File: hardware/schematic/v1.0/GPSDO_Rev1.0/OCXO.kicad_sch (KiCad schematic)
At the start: 47 parts, among them U10 SN74LVC1T45DBVR, U2 LMK1C1103PWR, U3 TMP117AIDRVR, U5 OCXO_20x20mm, U7 OCXO_25.4x25.4mm, U8 REF5040, U9 OPA388IDR

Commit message: sch update
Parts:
- C1, C16, C18, C22, C24, C4, C5: symbol GPSDO_Rev1.0:C -> GPSDO_Rev1.0:C__C_0402_1005Metric
- C11: footprint Capacitor_SMD:C_0402_1005Metric -> GPSDO_Rev1.0:C_0402_1005Metric; symbol Device:C -> GPSDO_Rev1.0:C__C_0402_1005Metric
- C56, C57, C58: footprint Capacitor_SMD:C_0603_1608Metric -> GPSDO_Rev1.0:C_0603_1608Metric; symbol Device:C -> GPSDO_Rev1.0:C
- R12, R13, R15, R16, R35, R37, R4: symbol GPSDO_Rev1.0:R -> GPSDO_Rev1.0:R__R_0402_1005Metric
- R28, R29: footprint Resistor_SMD:R_0603_1608Metric -> GPSDO_Rev1.0:R_0603_1608Metric; symbol Device:R -> GPSDO_Rev1.0:R
- R5: symbol GPSDO_Rev1.0:R -> GPSDO_Rev1.0:R__R_0805_2012Metric
- R6: symbol GPSDO_Rev1.0:R -> GPSDO_Rev1.0:R__C_0603_1608Metric
- TP1, TP2: footprint TestPoint:TestPoint_Pad_D1.0mm -> GPSDO_Rev1.0:TestPoint_Pad_D1.0mm; symbol Connector:TestPoint -> GPSDO_Rev1.0:TestPoint
- U8: footprint JLCImport:REF5040 -> GPSDO_Rev1.0:REF5040; symbol JLCImport:REF5040 -> GPSDO_Rev1.0:REF5040

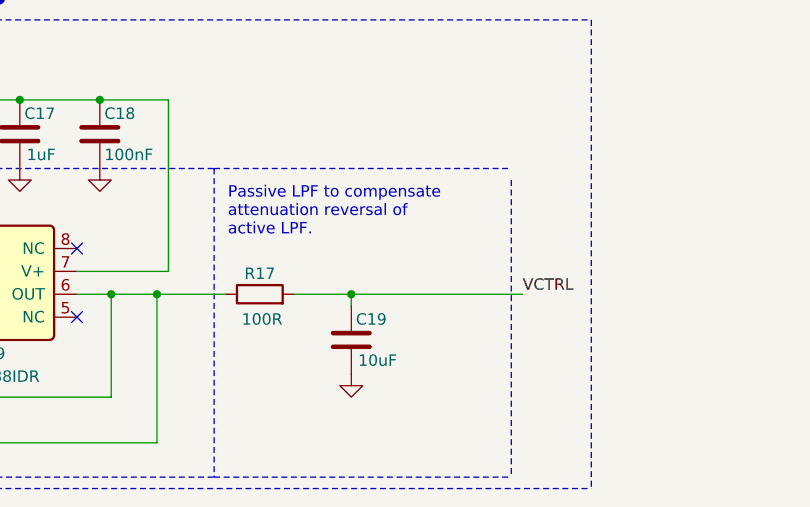
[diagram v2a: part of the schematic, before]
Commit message: sch update
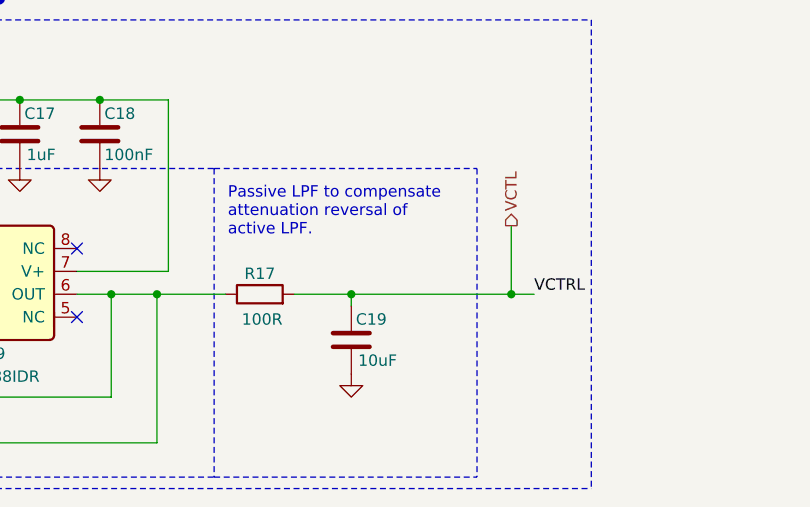
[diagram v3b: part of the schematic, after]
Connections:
- net VCTRL renamed VCTL
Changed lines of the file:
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@@
+	)
+	(junction
+		(at 246.38 35.56)
+		(diameter 0)
+		(color 0 0 0 0)
+	)
+	(junction
+		(at 78.74 111.76)
+		(diameter 0)
+		(color 0 0 0 0)
+	)
+	(junction
+		(at 67.31 111.76)
+		(diameter 0)
+		(color 0 0 0 0)
+	)
+	(junction
+		(at 205.74 44.45)
+		(diameter 0)
+		(color 0 0 0 0)
+	)
+	(junction
+		(at 72.39 173.99)
+		(diameter 0)
+		(color 0 0 0 0)
+	)
+	(junction
+		(at 120.65 173.99)
+		(diameter 0)
+		(color 0 0 0 0)
+	)
+	(junction
+		(at 201.93 57.15)
+		(diameter 0)
+		(color 0 0 0 0)
+	)
+	(junction
+		(at 83.82 50.8)
+		(diameter 0)
+		(color 0 0 0 0)
+	)
+	(junction
+		(at 142.24 111.76)
+		(diameter 0)
+		(color 0 0 0 0)
+	)
+	(junction
+		(at 92.71 111.76)
+		(diameter 0)
+		(color 0 0 0 0)
+	)
+	(junction
+		(at 165.1 173.99)
+		(diameter 0)
+		(color 0 0 0 0)
+	)
+	(junction
+		(at 87.63 173.99)
+		(diameter 0)
+		(color 0 0 0 0)
+	)
+	(junction
+		(at 110.49 152.4)
+		(diameter 0)
+		(color 0 0 0 0)
+	)
+	(junction
+		(at 246.38 46.99)
+		(diameter 0)
+		(color 0 0 0 0)
+	)
+	(junction
+		(at 46.99 50.8)
+		(diameter 0)
+		(color 0 0 0 0)
+	)
+	(junction
+		(at 138.43 102.87)
+		(diameter 0)
+		(color 0 0 0 0)
+	)
+	(junction
+		(at 129.54 111.76)
+		(diameter 0)
+		(color 0 0 0 0)
+	)
+	(junction
+		(at 157.48 97.79)
+		(diameter 0)
+		(color 0 0 0 0)
+	)
+	(junction
+		(at 134.62 111.76)
+		(diameter 0)
+		(color 0 0 0 0)
+	)
+	(junction
+		(at 125.73 173.99)
+		(diameter 0)
+		(color 0 0 0 0)
+	)
+	(junction
+		(at 198.12 44.45)
+		(diameter 0)
+		(color 0 0 0 0)
+	)
+	(junction
+		(at 25.4 173.99)
+		(diameter 0)
+		(color 0 0 0 0)
+	)
+	(junction
+		(at 157.48 106.68)
+		(diameter 0)
+		(color 0 0 0 0)
+	)
+	(junction
+		(at 49.53 151.13)
+		(diameter 0)
+		(color 0 0 0 0)
+	)
+	(junction
+		(at 205.74 57.15)
+		(diameter 0)
+		(color 0 0 0 0)
 	)
 	(junction
 		(at 147.32 173.99)
-		(diameter 0)
-		(color 0 0 0 0)
-	)
-	(junction
-		(at 246.38 35.56)
-		(diameter 0)
-		(color 0 0 0 0)
-	)
-	(junction
-		(at 78.74 111.76)
-		(diameter 0)
-		(color 0 0 0 0)
-	)
-	(junction
-		(at 67.31 111.76)
-		(diameter 0)
-		(color 0 0 0 0)
-	)
-	(junction
-		(at 205.74 44.45)
-		(diameter 0)
-		(color 0 0 0 0)
-	)
-	(junction
-		(at 72.39 173.99)
-		(diameter 0)
-		(color 0 0 0 0)
-	)
-	(junction
-		(at 120.65 173.99)
-		(diameter 0)
-		(color 0 0 0 0)
-	)
-	(junction
-		(at 201.93 57.15)
-		(diameter 0)
-		(color 0 0 0 0)
-	)
-	(junction
-		(at 83.82 50.8)
-		(diameter 0)
-		(color 0 0 0 0)
-	)
-	(junction
-		(at 142.24 111.76)
-		(diameter 0)
-		(color 0 0 0 0)
-	)
-	(junction
-		(at 92.71 111.76)
-		(diameter 0)
-		(color 0 0 0 0)
-	)
-	(junction
-		(at 87.63 173.99)
-		(diameter 0)
-		(color 0 0 0 0)
-	)
-	(junction
-		(at 110.49 152.4)
-		(diameter 0)
-		(color 0 0 0 0)
-	)
-	(junction
-		(at 246.38 46.99)
-		(diameter 0)
-		(color 0 0 0 0)
-	)
-	(junction
-		(at 46.99 50.8)
-		(diameter 0)
-		(color 0 0 0 0)
-	)
-	(junction
-		(at 138.43 102.87)
-		(diameter 0)
-		(color 0 0 0 0)
-	)
-	(junction
-		(at 129.54 111.76)
-		(diameter 0)
-		(color 0 0 0 0)
-	)
-	(junction
-		(at 157.48 97.79)
-		(diameter 0)
-		(color 0 0 0 0)
-	)
-	(junction
-		(at 134.62 111.76)
-		(diameter 0)
-		(color 0 0 0 0)
-	)
-	(junction
-		(at 125.73 173.99)
-		(diameter 0)
-		(color 0 0 0 0)
-	)
-	(junction
-		(at 198.12 44.45)
-		(diameter 0)
-		(color 0 0 0 0)
-	)
-	(junction
-		(at 25.4 173.99)
-		(diameter 0)
-		(color 0 0 0 0)
-	)
-	(junction
-		(at 157.48 106.68)
-		(diameter 0)
-		(color 0 0 0 0)
-	)
-	(junction
-		(at 49.53 151.13)
-		(diameter 0)
-		(color 0 0 0 0)
-	)
-	(junction
-		(at 205.74 57.15)
 		(diameter 0)
 		(color 0 0 0 0)
@@
 		)
 	)
-	(polyline
-		(pts
-			(xy 132.08 194.31) (xy 165.1 194.31)
+	(wire
+		(pts
+			(xy 165.1 166.37) (xy 165.1 173.99)
+		)
+		(stroke
+			(width 0)
+			(type default)
+		)
+	)
+	(polyline
+		(pts
+			(xy 132.08 194.31) (xy 161.29 194.31)
 		)
 		(stroke
@@
 	(wire
 		(pts
+			(xy 165.1 173.99) (xy 167.64 173.99)
+		)
+		(stroke
+			(width 0)
+			(type default)
+		)
+	)
+	(wire
+		(pts
 			(xy 201.93 116.84) (xy 219.71 116.84)
 		)
@@
 	(polyline
 		(pts
-			(xy 132.08 160.02) (xy 165.1 160.02)
+			(xy 132.08 160.02) (xy 161.29 160.02)
 		)
 		(stroke
@@
 	(polyline
 		(pts
-			(xy 165.1 161.29) (xy 165.1 194.31)
+			(xy 161.29 160.02) (xy 161.29 194.31)
 		)
 		(stroke
@@
 	(wire
 		(pts
-			(xy 147.32 173.99) (xy 166.37 173.99)
+			(xy 147.32 173.99) (xy 165.1 173.99)
 		)
 		(stroke
@@
 	)
 	(label "VCTRL"
-		(at 166.37 173.99 0)
+		(at 167.64 173.99 0)
 		(effects
 			(font
@@
 		(effects
 			(font
+				(size 1.27 1.27)
+			)
+			(justify left)
+		)
+	)
+	(hierarchical_label "VCTL"
+		(shape output)
+		(at 165.1 166.37 90)
+		(effects
+			(font
